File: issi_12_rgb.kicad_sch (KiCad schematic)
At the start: 16 parts, among them U1 IS31FL3236A

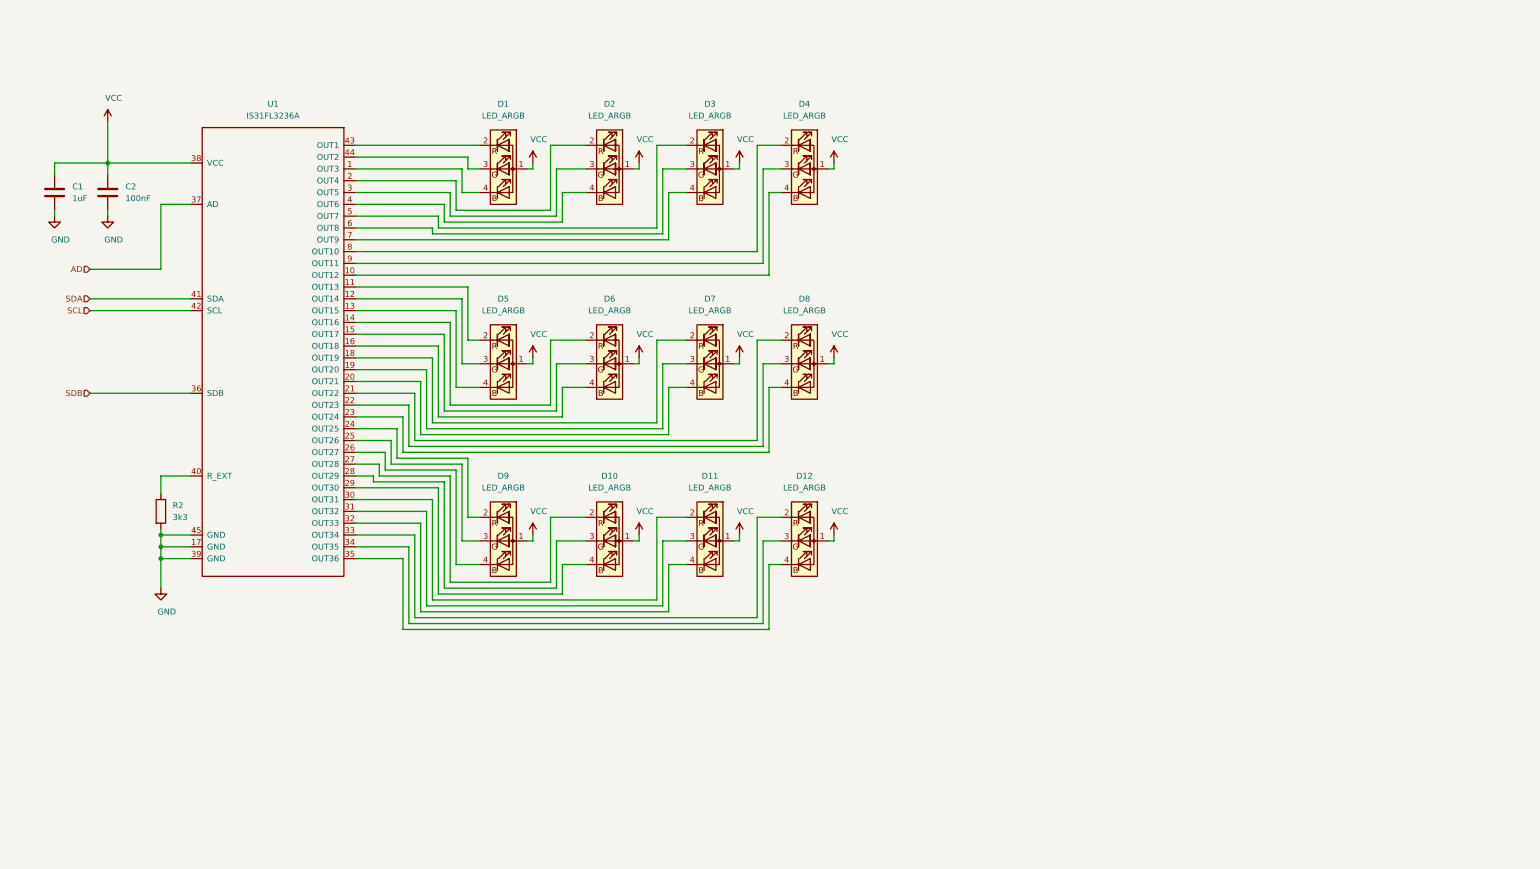
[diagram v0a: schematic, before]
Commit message: gregdavill: Initial commit of new badge design
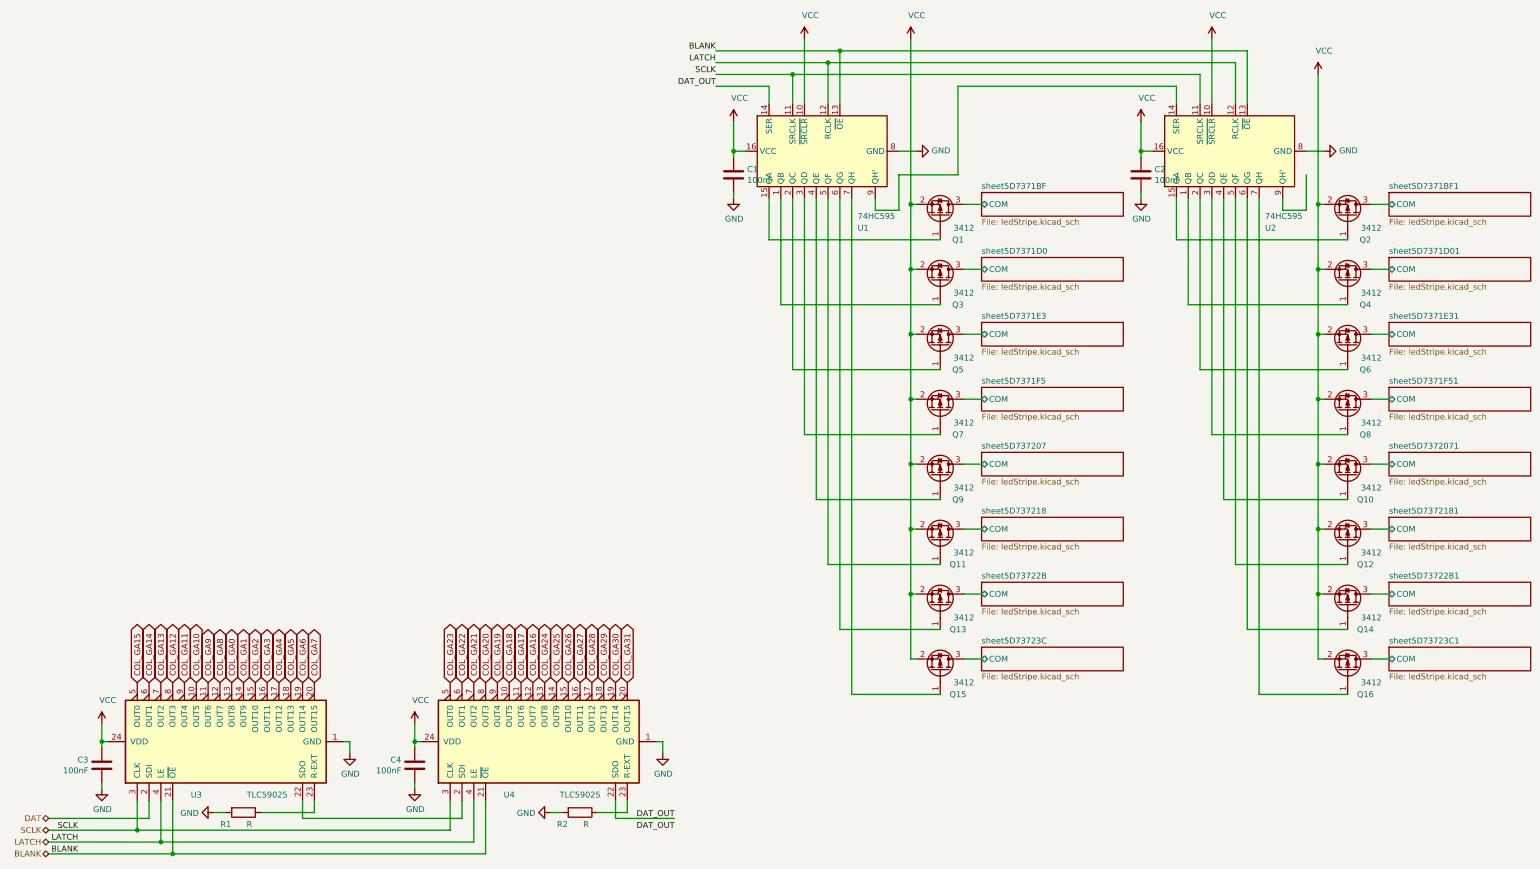
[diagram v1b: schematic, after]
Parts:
- removed D1, D10, D11, D12, D2, D3, D4, D5, D6, D7, D8, D9: LED_ARGB, Opto:ARGB-1x1mm, symbol Device:LED_ARGB
- removed U1: IS31FL3236A, SMD_Semiconductors:QFN-44_EP_5x5_Pitch0.4mm, symbol is31fl3236a:IS31FL3236A
- added C3, C4: 100nF, Capacitor_SMD:C_0603_1608Metric, symbol Device:C
- added Q1, Q10, Q11, Q12, Q13, Q14, Q15, Q16, Q2, Q3, Q4, Q5, Q6, Q7, Q8, Q9: 3412, Package_TO_SOT_SMD:SOT-883, symbol Device:Q_PMOS_GSD
- added R1: R, Resistor_SMD:R_0603_1608Metric, symbol Device:R
- added U1, U2: 74HC595, Package_SO:TSSOP-16_4.4x5mm_P0.65mm, symbol 74xx:74HC595
- added U3, U4: TLC59025, Package_SO:SSOP-24_3.9x8.7mm_P0.635mm, symbol panel_r0.1-rescue:TLC59025-gkl_misc
- C1: value 1uF -> 100nF
- R2: value 3k3 -> R
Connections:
- net GND: now also C3.2, C4.2, R1.2, U1.8 (GND), U2.8 (GND), U3.1 (GND), U4.1 (GND)
- net VCC: now also C3.1, C4.1, Q1.2 (S), Q10.2 (S), Q11.2 (S), Q12.2 (S), Q13.2 (S), Q14.2 (S), Q15.2 (S), Q16.2 (S), Q2.2 (S), Q3.2 (S), Q4.2 (S), Q5.2 (S), Q6.2 (S), Q7.2 (S), Q8.2 (S), Q9.2 (S), U1.10 (~SRCLR), U1.16 (VCC), U2.10 (~SRCLR), U2.16 (VCC), U3.24 (VDD), U4.24 (VDD)
- net at R2.1: now also U4.23 (R-EXT)
- new net: Q6.1 (G), U2.2 (QC)
- new net: U3.22 (SDO), U4.2 (SDI)
- new net: Q8.1 (G), U2.3 (QD)
- new net: Q5.1 (G), U1.2 (QC)
- new net: R1.1, U3.23 (R-EXT)
- new net: Q4.1 (G), U2.1 (QB)
- new net: U1.9 (QH'), U2.14 (SER)
- new net: Q2.1 (G), U2.15 (QA)
- new net: Q10.1 (G), U2.4 (QE)
- new net: Q12.1 (G), U2.5 (QF)
- new net: Q14.1 (G), U2.6 (QG)
- new net: Q16.1 (G), U2.7 (QH)
- new net: Q3.1 (G), U1.1 (QB)
- new net: Q1.1 (G), U1.15 (QA)
- new net: Q7.1 (G), U1.3 (QD)
- new net: Q9.1 (G), U1.4 (QE)
- new net: Q11.1 (G), U1.5 (QF)
- new net: Q13.1 (G), U1.6 (QG)
- new net: Q15.1 (G), U1.7 (QH)
- new net BLANK: U1.13 (~OE), U2.13 (~OE), U3.21 (~OE), U4.21 (~OE)
- new net COL_GA0: U3.13 (OUT8)
- new net COL_GA1: U3.14 (OUT9)
- new net COL_GA10: U3.10 (OUT5)
- new net COL_GA11: U3.9 (OUT4)
- new net COL_GA12: U3.8 (OUT3)
- new net COL_GA13: U3.7 (OUT2)
- new net COL_GA14: U3.6 (OUT1)
- new net COL_GA15: U3.5 (OUT0)
- new net COL_GA16: U4.12 (OUT7)
- new net COL_GA17: U4.11 (OUT6)
- new net COL_GA18: U4.10 (OUT5)
- new net COL_GA19: U4.9 (OUT4)
- new net COL_GA2: U3.15 (OUT10)
- new net COL_GA20: U4.8 (OUT3)
- new net COL_GA21: U4.7 (OUT2)
- new net COL_GA22: U4.6 (OUT1)
- new net COL_GA23: U4.5 (OUT0)
- new net COL_GA24: U4.13 (OUT8)
- new net COL_GA25: U4.14 (OUT9)
- new net COL_GA26: U4.15 (OUT10)
- new net COL_GA27: U4.16 (OUT11)
- new net COL_GA28: U4.17 (OUT12)
- new net COL_GA29: U4.18 (OUT13)
- new net COL_GA3: U3.16 (OUT11)
- new net COL_GA30: U4.19 (OUT14)
- new net COL_GA31: U4.20 (OUT15)
- new net COL_GA4: U3.17 (OUT12)
- new net COL_GA5: U3.18 (OUT13)
- new net COL_GA6: U3.19 (OUT14)
- new net COL_GA7: U3.20 (OUT15)
- new net COL_GA8: U3.12 (OUT7)
- new net COL_GA9: U3.11 (OUT6)
- new net DAT: U3.2 (SDI)
- new net DAT_OUT: U1.14 (SER), U4.22 (SDO)
- new net LATCH: U1.12 (RCLK), U2.12 (RCLK), U3.4 (LE), U4.4 (LE)
- new net SCLK: U1.11 (SRCLK), U2.11 (SRCLK), U3.3 (CLK), U4.3 (CLK)
- new net sheet5D7371BF/COM: Q1.3 (D)
- new net sheet5D7371BF1/COM: Q2.3 (D)
- new net sheet5D7371D0/COM: Q3.3 (D)
- new net sheet5D7371D01/COM: Q4.3 (D)
- new net sheet5D7371E3/COM: Q5.3 (D)
- new net sheet5D7371E31/COM: Q6.3 (D)
- new net sheet5D7371F5/COM: Q7.3 (D)
- new net sheet5D7371F51/COM: Q8.3 (D)
- new net sheet5D737207/COM: Q9.3 (D)
- new net sheet5D7372071/COM: Q10.3 (D)
- new net sheet5D737218/COM: Q11.3 (D)
- new net sheet5D7372181/COM: Q12.3 (D)
- new net sheet5D73722B/COM: Q13.3 (D)
- new net sheet5D73722B1/COM: Q14.3 (D)
- new net sheet5D73723C/COM: Q15.3 (D)
- new net sheet5D73723C1/COM: Q16.3 (D)
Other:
- added sheet sheet5D7371BF (ledStripe.kicad_sch)
- added sheet sheet5D7371BF1 (ledStripe.kicad_sch)
- added sheet sheet5D7371D0 (ledStripe.kicad_sch)
- added sheet sheet5D7371D01 (ledStripe.kicad_sch)
- added sheet sheet5D7371E3 (ledStripe.kicad_sch)
- added sheet sheet5D7371E31 (ledStripe.kicad_sch)
- added sheet sheet5D7371F5 (ledStripe.kicad_sch)
- added sheet sheet5D7371F51 (ledStripe.kicad_sch)
- added sheet sheet5D737207 (ledStripe.kicad_sch)
- added sheet sheet5D7372071 (ledStripe.kicad_sch)
- added sheet sheet5D737218 (ledStripe.kicad_sch)
- added sheet sheet5D7372181 (ledStripe.kicad_sch)
- added sheet sheet5D73722B (ledStripe.kicad_sch)
- added sheet sheet5D73722B1 (ledStripe.kicad_sch)
- added sheet sheet5D73723C (ledStripe.kicad_sch)
- added sheet sheet5D73723C1 (ledStripe.kicad_sch)
